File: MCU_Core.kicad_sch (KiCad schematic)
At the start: 16 parts, among them U1 STM32F405RGTx

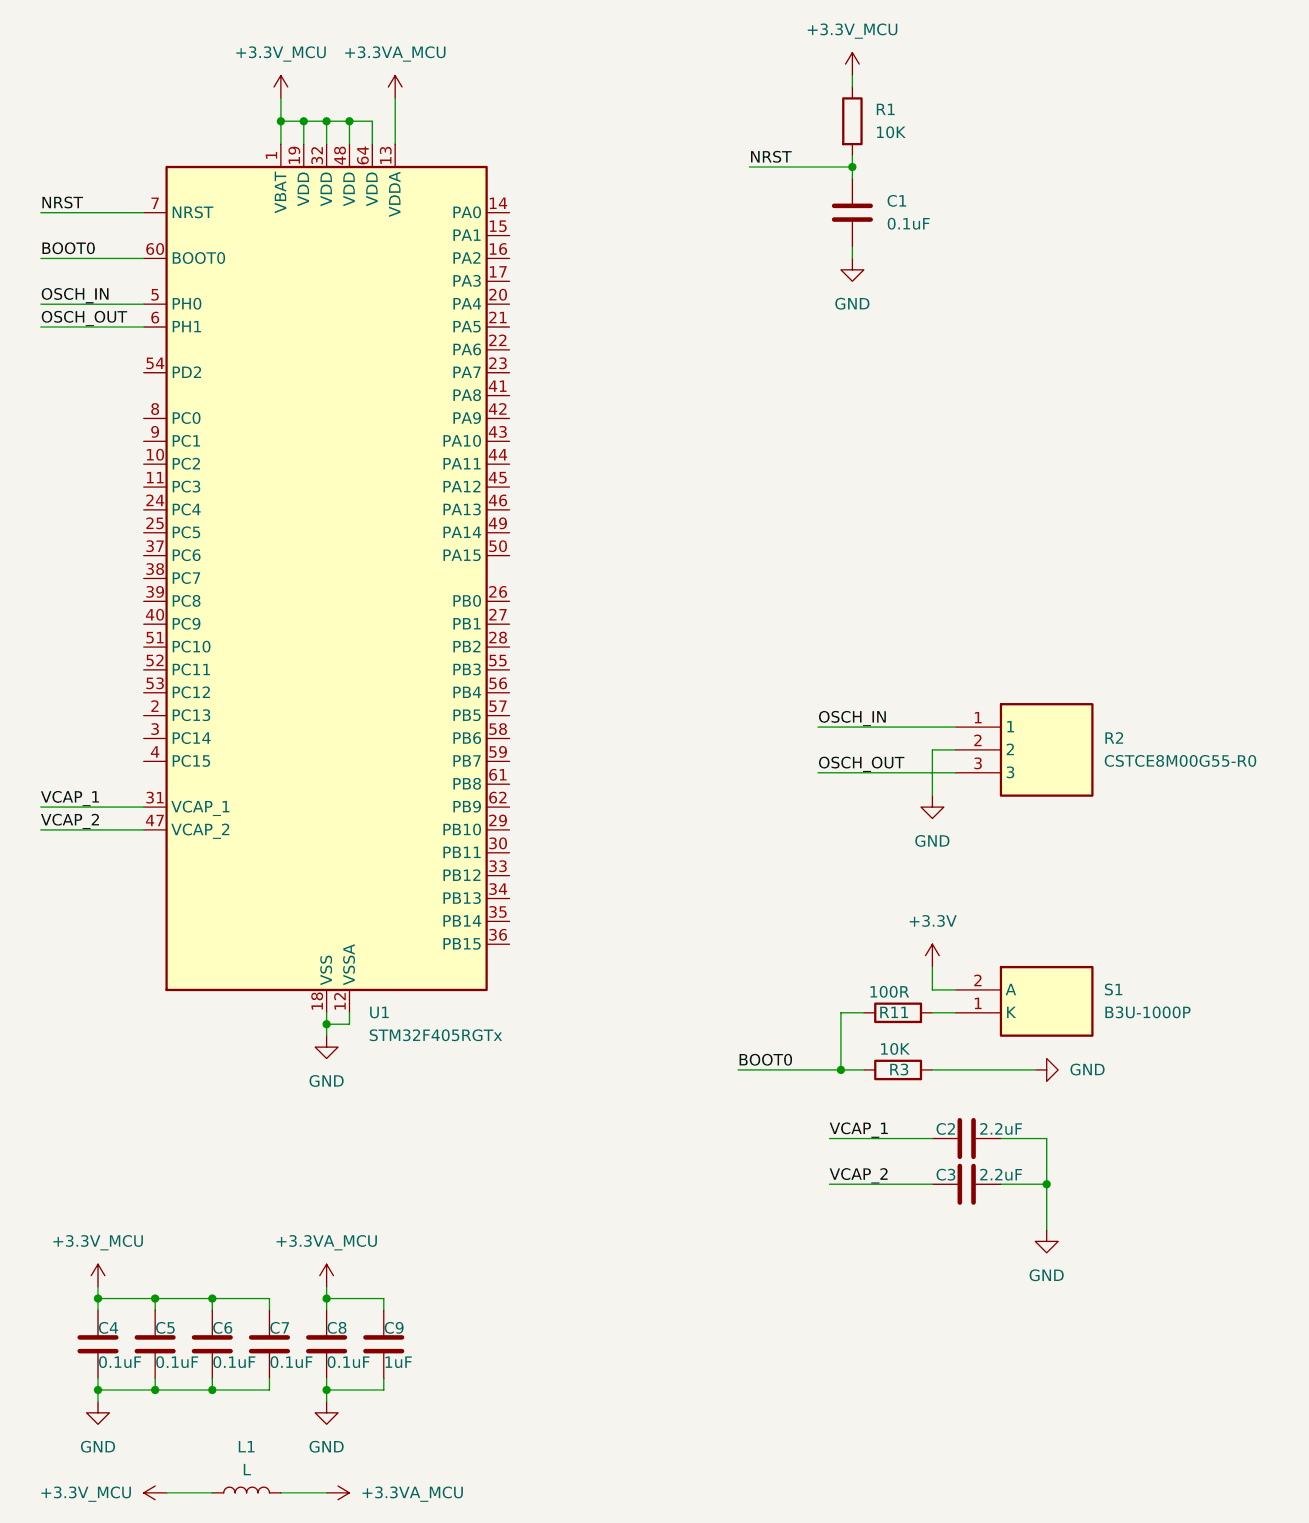
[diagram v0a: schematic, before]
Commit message: Update SCH
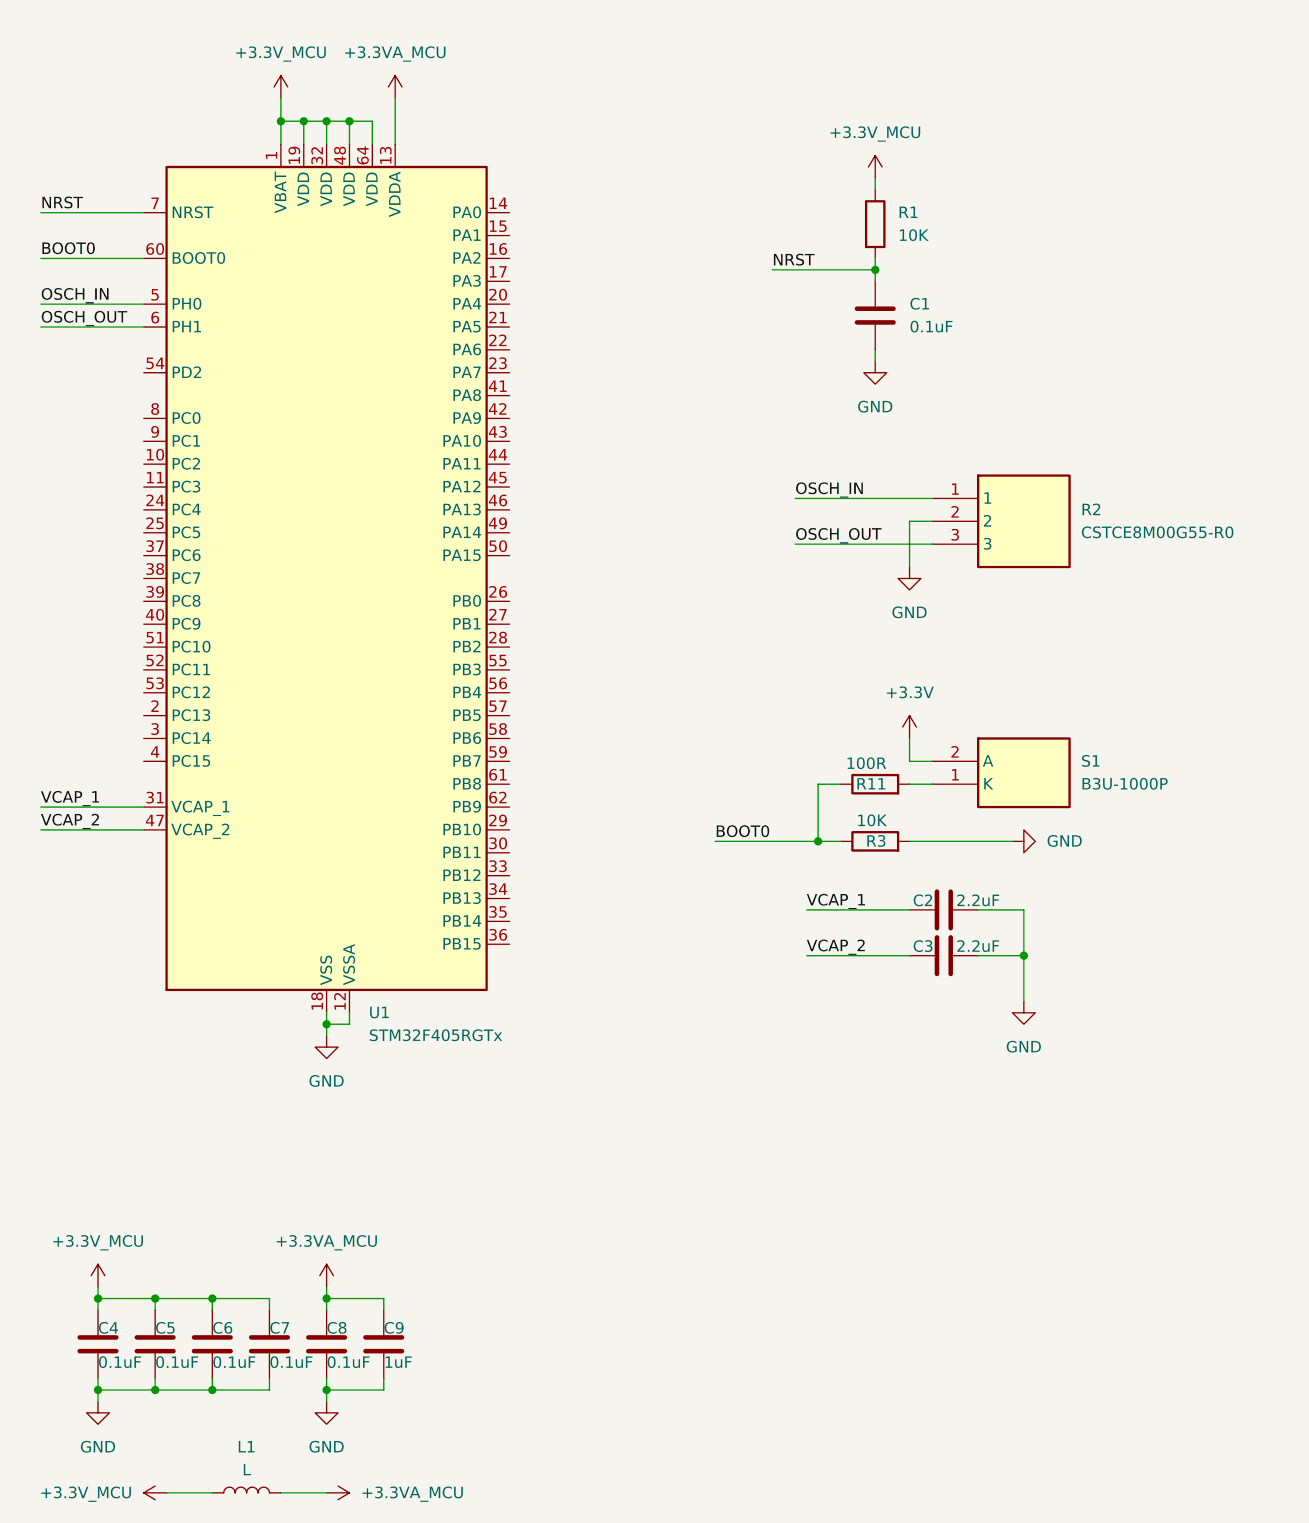
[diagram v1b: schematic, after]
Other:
- moved on the sheet: C1, C2, C3, R1, R11, R2, R3, S1
